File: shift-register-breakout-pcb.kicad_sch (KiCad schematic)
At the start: 29 parts, among them J1 Conn_01x04_Socket, J2 Conn_01x08_Socket, J3 Conn_01x08_Socket, J4 Conn_01x08_Socket, J5 Conn_01x08_Socket, J6 Conn_01x03_Socket, J7 vik-module-connector, J8 Conn_01x04_Socket

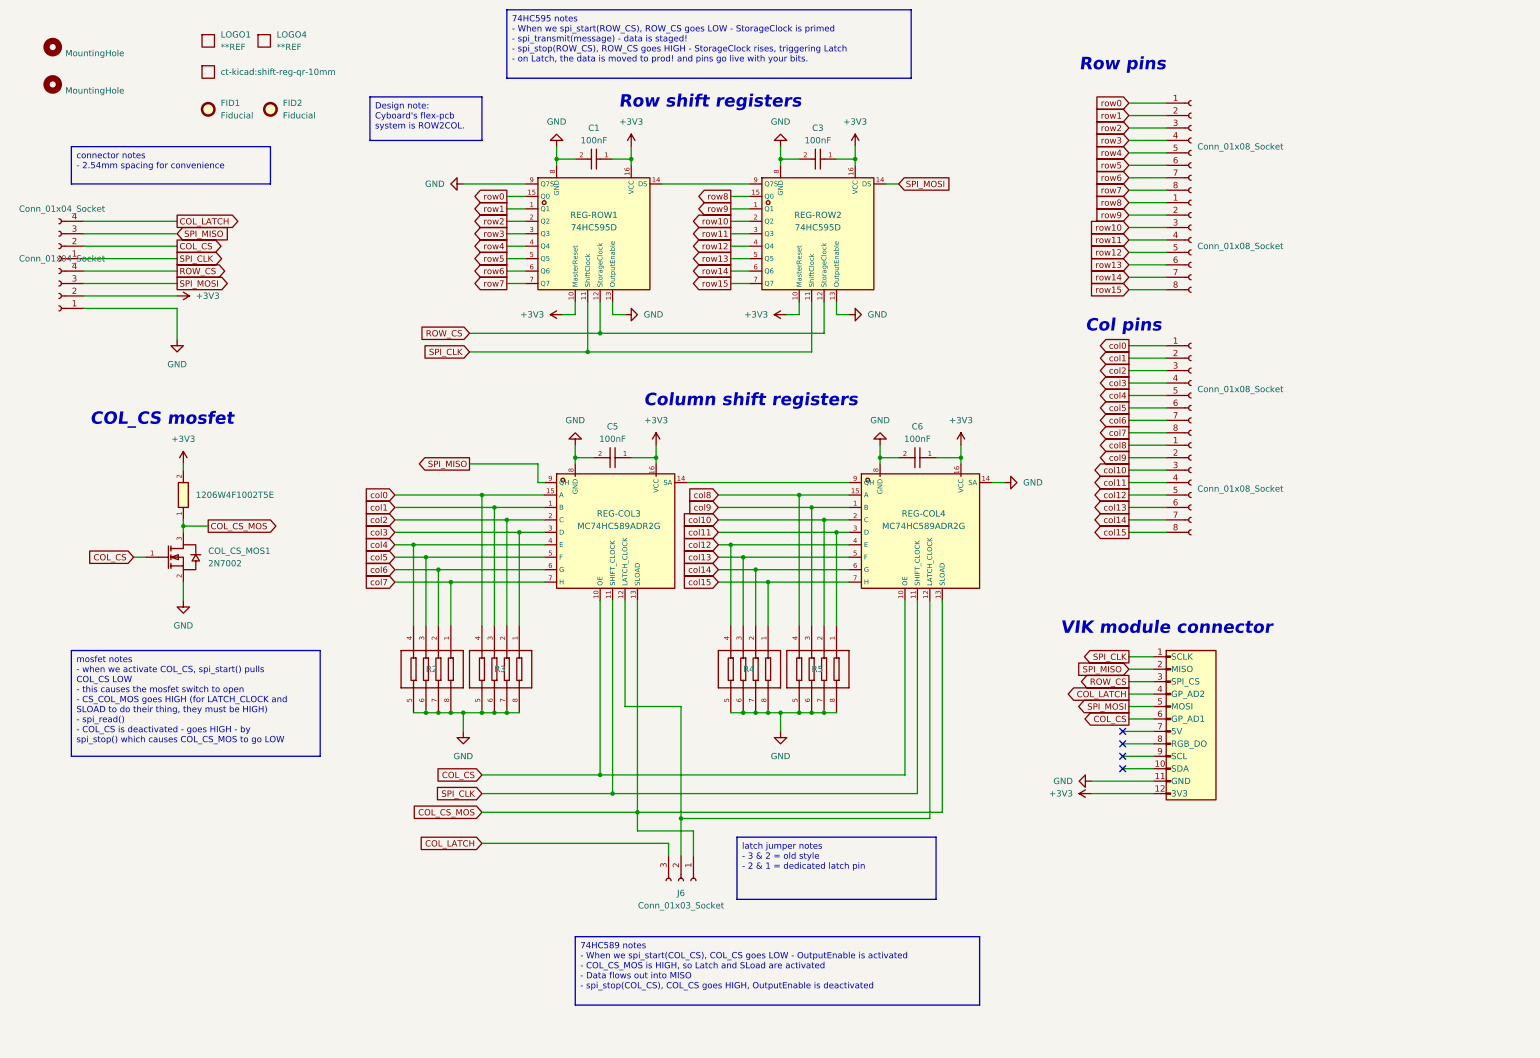
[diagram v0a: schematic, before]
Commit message: almost done readme
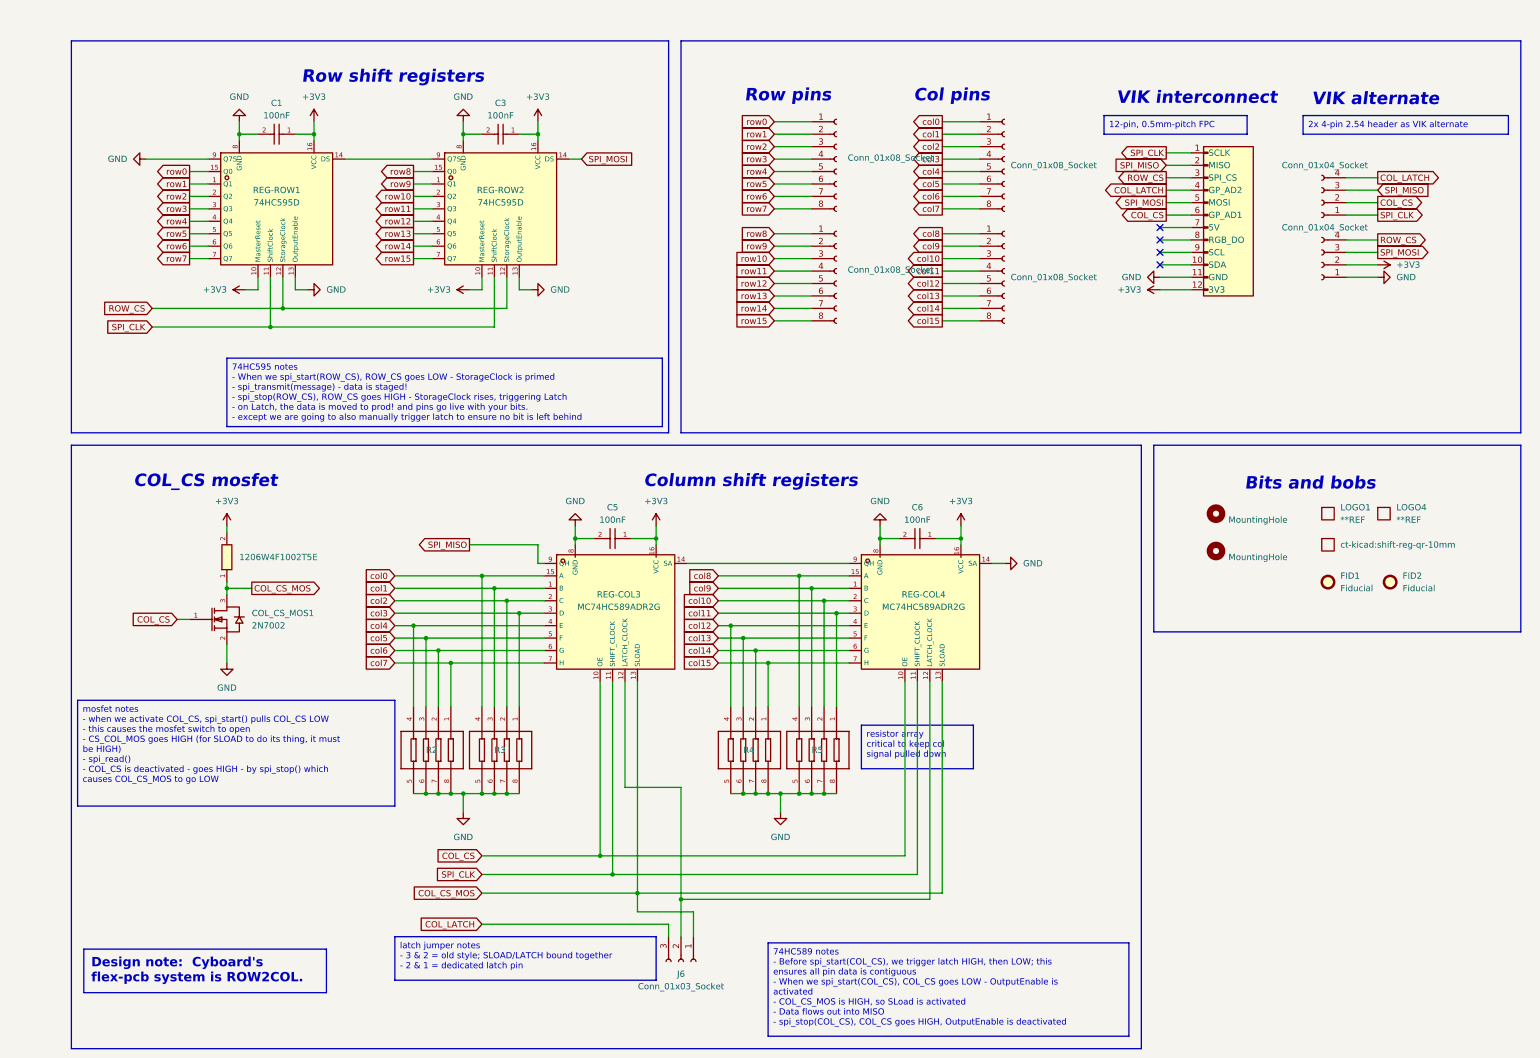
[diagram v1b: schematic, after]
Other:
- note added: "Bits and bobs"
- note added: "VIK alternate"
- note added: "VIK interconnect"
- note removed: "VIK module connector"
- moved on the sheet: C1, C3, C5, C6, COL_CS_MOS1, FID1, FID2, J6, LOGO1, LOGO4, R2, R3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
